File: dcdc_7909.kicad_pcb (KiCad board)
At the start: 2 copper layers, 40 x 27 mm, 50 parts, among them J1 V_IN, J2 G_IN, J3 RFShield_OnePiece, J4 +10V, J5 G_OUT, J6 -10V, U1 LM2940-SOT223-15, U2 LT3471, U3 LT3045xMSE, U4 LT3094xMSE

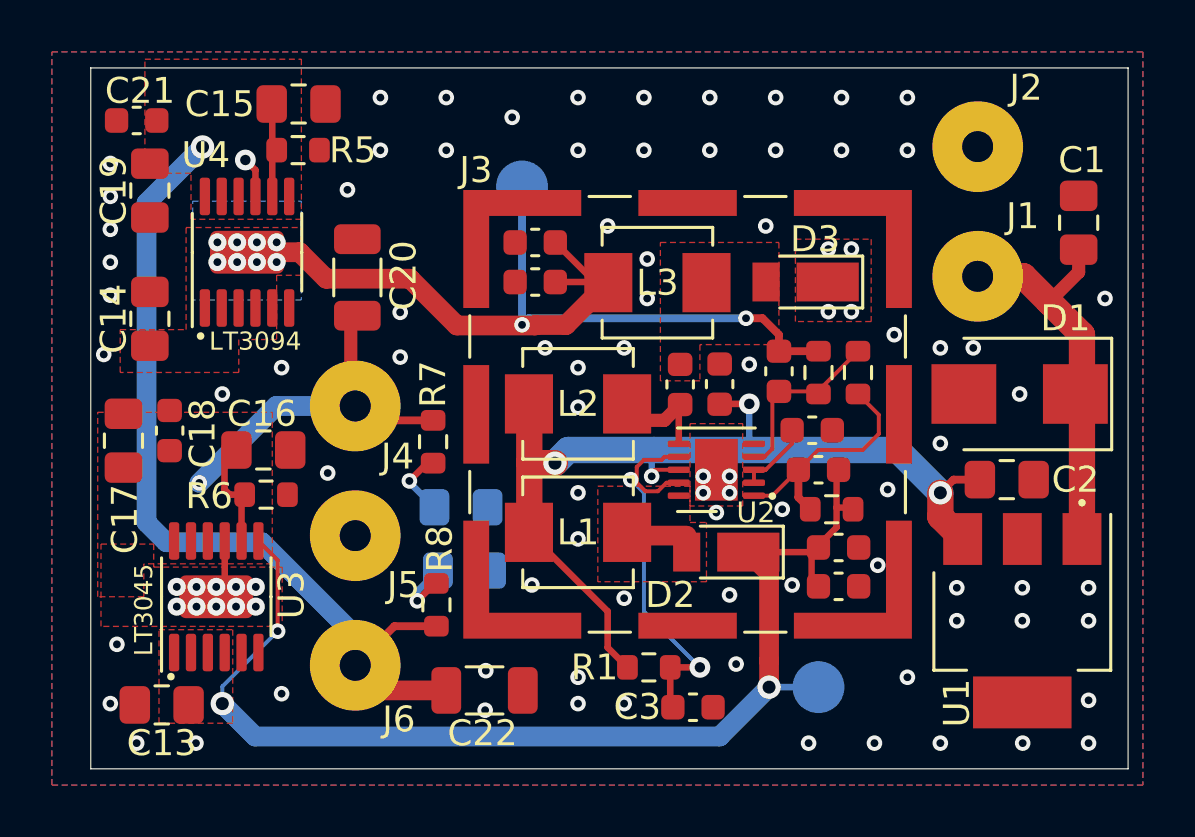
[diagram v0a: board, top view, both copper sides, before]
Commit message: WIP on version 2.1, routing mostly done.
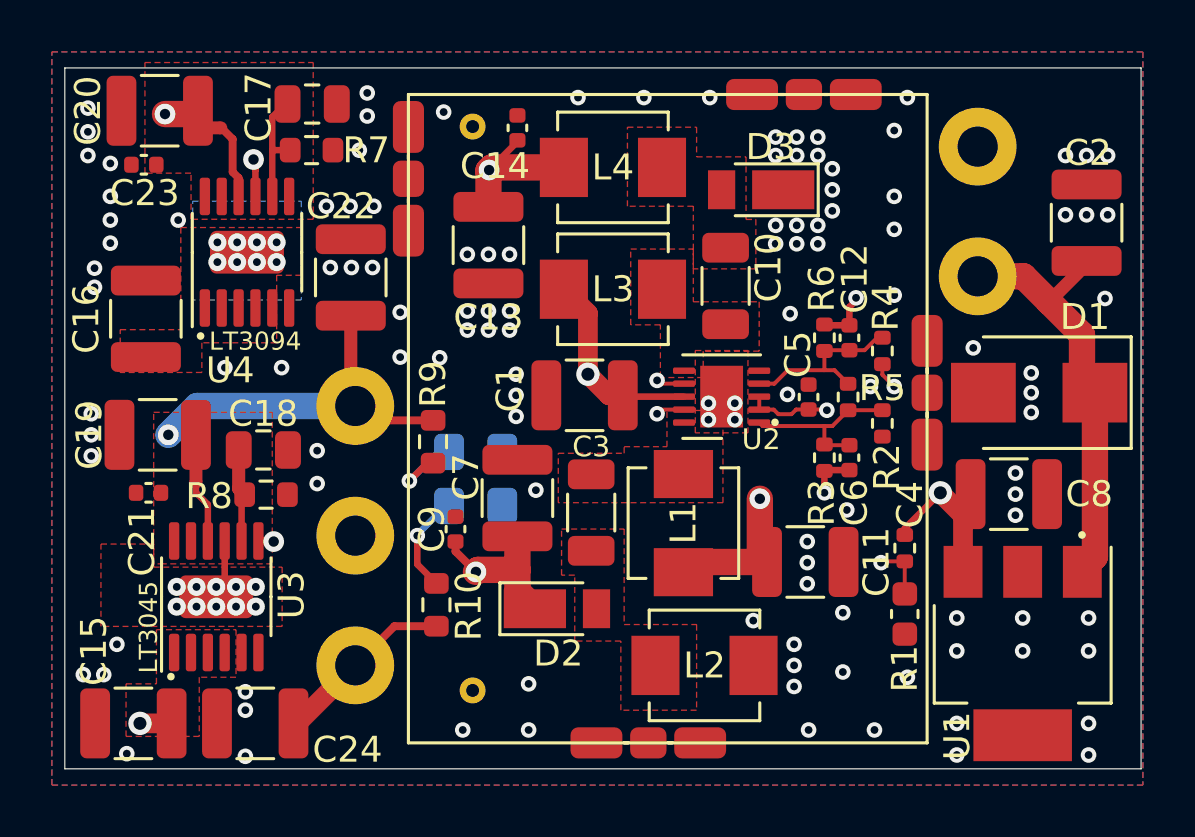
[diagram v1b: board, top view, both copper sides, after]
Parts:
- added C3: 4u7, Capacitor_SMD:C_1206_3216Metric, F.Cu at (98.3, 71.1)
- added C8: 22u, Capacitor_SMD:C_1210_3225Metric, F.Cu at (114.4, 70.4)
- added J4: RFShield_Clip, marcin_library:S0971-46R, F.Cu at (100.5, 80.0)
- added J5: RFShield_Clip, marcin_library:S0971-46R, F.Cu at (91.2, 58.2)
- added J6: RFShield_Clip, marcin_library:S0971-46R, F.Cu at (106.5, 55.0)
- added L2: 10u, Inductor_SMD:L_Vishay_IHLP-1616, F.Cu at (102.7, 77.0)
- added NT1: NetTie_2, NetTie:NetTie-2_SMD_Pad0.5mm, F.Cu at (83.1, 69.4)
- added NT2: NetTie_2, NetTie:NetTie-2_SMD_Pad0.5mm, F.Cu at (83.5, 56.3)
- added R2: DNP, Resistor_SMD:R_0402_1005Metric, F.Cu at (109.5, 67.7)
- added R4: DNP, Resistor_SMD:R_0402_1005Metric, F.Cu at (109.5, 64.9)
- C1: renamed from C2; footprint Capacitor_SMD:C_0805_2012Metric_Pad1.18x1.45mm_HandSolder -> Capacitor_SMD:C_1210_3225Metric
- C10: renamed from C8; value 10u -> 4u7; footprint Capacitor_SMD:C_0603_1608Metric -> Capacitor_SMD:C_1206_3216Metric
- C11: renamed from C9; value 10u -> 22u; footprint Capacitor_SMD:C_0603_1608Metric -> Capacitor_SMD:C_1210_3225Metric
- C12: renamed from C10; footprint Capacitor_SMD:C_0603_1608Metric -> Capacitor_SMD:C_0402_1005Metric
- C13: renamed from C11; value 10u -> 22u; footprint Capacitor_SMD:C_0603_1608Metric -> Capacitor_SMD:C_1210_3225Metric
- C14: renamed from C12; footprint Capacitor_SMD:C_0603_1608Metric -> Capacitor_SMD:C_0402_1005Metric
- C15: renamed from C13; value 10u -> 22u; footprint Capacitor_SMD:C_0805_2012Metric_Pad1.18x1.45mm_HandSolder -> Capacitor_SMD:C_1210_3225Metric
- C16: renamed from C14; value 10u -> 22u; footprint Capacitor_SMD:C_0805_2012Metric_Pad1.18x1.45mm_HandSolder -> Capacitor_SMD:C_1210_3225Metric
- C17: renamed from C15; footprint Capacitor_SMD:C_0805_2012Metric_Pad1.18x1.45mm_HandSolder -> Capacitor_SMD:C_0805_2012Metric
- C18: renamed from C16; footprint Capacitor_SMD:C_0805_2012Metric_Pad1.18x1.45mm_HandSolder -> Capacitor_SMD:C_0805_2012Metric
- C19: renamed from C17; value 10u -> 22u; footprint Capacitor_SMD:C_0805_2012Metric_Pad1.18x1.45mm_HandSolder -> Capacitor_SMD:C_1210_3225Metric
- C2: renamed from C1; footprint Capacitor_SMD:C_0805_2012Metric_Pad1.18x1.45mm_HandSolder -> Capacitor_SMD:C_1210_3225Metric
- C20: renamed from C19; value 10u -> 22u; footprint Capacitor_SMD:C_0805_2012Metric_Pad1.18x1.45mm_HandSolder -> Capacitor_SMD:C_1210_3225Metric
- C21: renamed from C18; footprint Capacitor_SMD:C_0603_1608Metric -> Capacitor_SMD:C_0402_1005Metric
- C22: renamed from C20; footprint Capacitor_SMD:C_1206_3216Metric -> Capacitor_SMD:C_1210_3225Metric
- C23: renamed from C21; footprint Capacitor_SMD:C_0603_1608Metric -> Capacitor_SMD:C_0402_1005Metric
- C24: renamed from C22; footprint Capacitor_SMD:C_1206_3216Metric -> Capacitor_SMD:C_1210_3225Metric
- C5: renamed from C4; footprint Capacitor_SMD:C_0603_1608Metric -> Capacitor_SMD:C_0402_1005Metric
- C6: renamed from C5; footprint Capacitor_SMD:C_0603_1608Metric -> Capacitor_SMD:C_0402_1005Metric
- C7: renamed from C6; value 10u -> 22u; footprint Capacitor_SMD:C_0603_1608Metric -> Capacitor_SMD:C_1210_3225Metric
- C9: renamed from C7; footprint Capacitor_SMD:C_0603_1608Metric -> Capacitor_SMD:C_0402_1005Metric
- D1: value SM6T15A -> P6SMB20A
- J1, J2: footprint Connector_Wire:SolderWirePad_1x01_Drill1.2mm -> Connector_Wire:SolderWire-0.75sqmm_1x01_D1.25mm_OD3.5mm
- J3: value RFShield_OnePiece -> RFShield_Clip; footprint RF_Shielding:Laird_Technologies_BMI-S-102_16.50x16.50mm -> marcin_library:S0971-46R
- J7: renamed from J4; footprint Connector_Wire:SolderWirePad_1x01_Drill1.2mm -> Connector_Wire:SolderWire-0.75sqmm_1x01_D1.25mm_OD3.5mm
- J8: renamed from J5; footprint Connector_Wire:SolderWirePad_1x01_Drill1.2mm -> Connector_Wire:SolderWire-0.75sqmm_1x01_D1.25mm_OD3.5mm
- J9: renamed from J6; footprint Connector_Wire:SolderWirePad_1x01_Drill1.2mm -> Connector_Wire:SolderWire-0.75sqmm_1x01_D1.25mm_OD3.5mm
- R1: footprint Resistor_SMD:R_0603_1608Metric -> Resistor_SMD:R_0402_1005Metric
- R3: renamed from R2; footprint Resistor_SMD:R_0603_1608Metric -> Resistor_SMD:R_0402_1005Metric
- R5: renamed from R3; footprint Resistor_SMD:R_0603_1608Metric -> Resistor_SMD:R_0402_1005Metric
- R6: renamed from R4; footprint Resistor_SMD:R_0603_1608Metric -> Resistor_SMD:R_0402_1005Metric
- TP1, TP2: footprint TestPoint:TestPoint_Pad_D2.0mm -> TestPoint:TestPoint_THTPad_D1.0mm_Drill0.5mm
- moved C1 16.6 mm to (98.0, 66.6), turned to 180 degrees
- moved C9 14.8 mm to (93.1, 71.8), turned to 90 degrees
- moved TP1 13.3 mm to (93.7, 78.0)
- moved C7 12.8 mm to (95.5, 70.6), turned to 90 degrees
- moved R1 10.9 mm to (110.4, 72.5), turned to -90 degrees
- moved J3 9.27 mm to (111.2, 66.5), turned to 90 degrees
- moved C24 8.93 mm to (85.3, 79.2), turned to 180 degrees
- moved C4 8.92 mm to (110.4, 75.0), turned to -90 degrees
- moved C11 7.61 mm to (106.6, 73.0), turned to 0 degrees
- moved D2 6.88 mm to (97.0, 74.8), turned to 0 degrees
- moved C14 5.98 mm to (95.5, 56.3), turned to 90 degrees
- moved L4 4.76 mm to (99.1, 57.8)
- moved L3 4.62 mm to (99.1, 62.5)
- moved C10 4.18 mm to (103.5, 62.4)
- moved L1 4.08 mm to (101.9, 71.5), turned to 90 degrees
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- renumbered C3 to C4, L2 to L3, L3 to L4, R8 to R10, R5 to R7, R6 to R8, R7 to R9
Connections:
- D2 pad 2: Net-(D2-Pad2) -> Net-(C3-Pad2)
- L1 pad 2: Net-(D2-Pad2) -> Net-(C3-Pad1)
- U2 pad 10: Net-(D2-Pad2) -> Net-(C3-Pad1)
- U3 pad 10: /+10V -> Net-(NT1-Pad1)
- U4 pad 10: /-10V -> Net-(NT2-Pad1)
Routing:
- net /+10.5V: track 46.1 -> 62.9 mm, vias 3 -> 4
- net Net-(C4-Pad1): track 15.3 -> 28.8 mm, vias 2 -> 3
- net Net-(C5-Pad1): track 2.90 -> 7.60 mm, vias 0 -> 2
- net Net-(C10-Pad1): track 3.82 -> 0.00 mm
- net /-10V: track 33.9 -> 37.5 mm
- net Net-(NT2-Pad1): track 0.00 -> 2.92 mm
- net Net-(C6-Pad2): track 9.39 -> 6.54 mm
- net Net-(NT1-Pad1): track 0.00 -> 2.46 mm
- net Net-(D2-Pad2): track 2.46 -> 0.00 mm
- net /-10.5V: track 38.3 -> 40.5 mm
- net Net-(D5-Pad1): track 2.51 -> 3.88 mm
- net Net-(C17-Pad1): track 3.57 -> 4.46 mm
- net Net-(C2-Pad1): track 15.3 -> 16.0 mm
- net Net-(C18-Pad1): track 4.01 -> 3.38 mm
- net Net-(D4-Pad2): track 2.61 -> 3.17 mm
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- added copper zone on In1.Cu, net GND
- added copper zone on In2.Cu, net GND
- added copper zone on F.Cu, net Net-(C10-Pad1)
- added copper zone on F.Cu, net Net-(C3-Pad1)
- added copper zone on F.Cu, net Net-(C3-Pad2)
- removed copper zone on F.Cu, net Net-(D2-Pad2)
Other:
- board size 40 x 27 mm -> 41.5 x 27 mm
- copper layers 2 -> 4
- board text added: "Alpine 7909 DC/DC v2.1 (c) M. Dymczyk 08.2023"
- board text removed: "Alpine 7909 DC/DC v2.0 (c) M. Dymczyk 07.2023"
